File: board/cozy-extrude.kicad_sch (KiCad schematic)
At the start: 7 parts, among them J1 RPi-Pico-Socket, J2 BME280, J3 PWM-Fan, J4 Heater-Switch, K1 HF46F_5-HS1, U1 ULN2003

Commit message: improved hf46f footprint and model
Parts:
- K1: footprint Hongfa-HF46F:HF46F_5-HS1 -> Hongfa-HF46F:HF46F
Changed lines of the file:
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@@
     (property "Reference" "K1" (id 0) (at 178.435 103.505 90))
     (property "Value" "HF46F_5-HS1" (id 1) (at 179.07 106.045 90))
-    (property "Footprint" "Hongfa-HF46F:HF46F_5-HS1" (id 2) (at 190.5 97.79 0)
+    (property "Footprint" "Hongfa-HF46F:HF46F" (id 2) (at 190.5 97.79 0)
       (effects (font (size 1.27 1.27)) hide)
     )
@@
     )
     (path "/e81af6a5-45c6-4d18-ac2c-2f6d6836f747"
-      (reference "K1") (unit 1) (value "HF46F_5-HS1") (footprint "Hongfa-HF46F:HF46F_5-HS1")
+      (reference "K1") (unit 1) (value "HF46F_5-HS1") (footprint "Hongfa-HF46F:HF46F")
     )
     (path "/a47ea3c8-3841-47fd-a5b3-6e9dc298f59d"

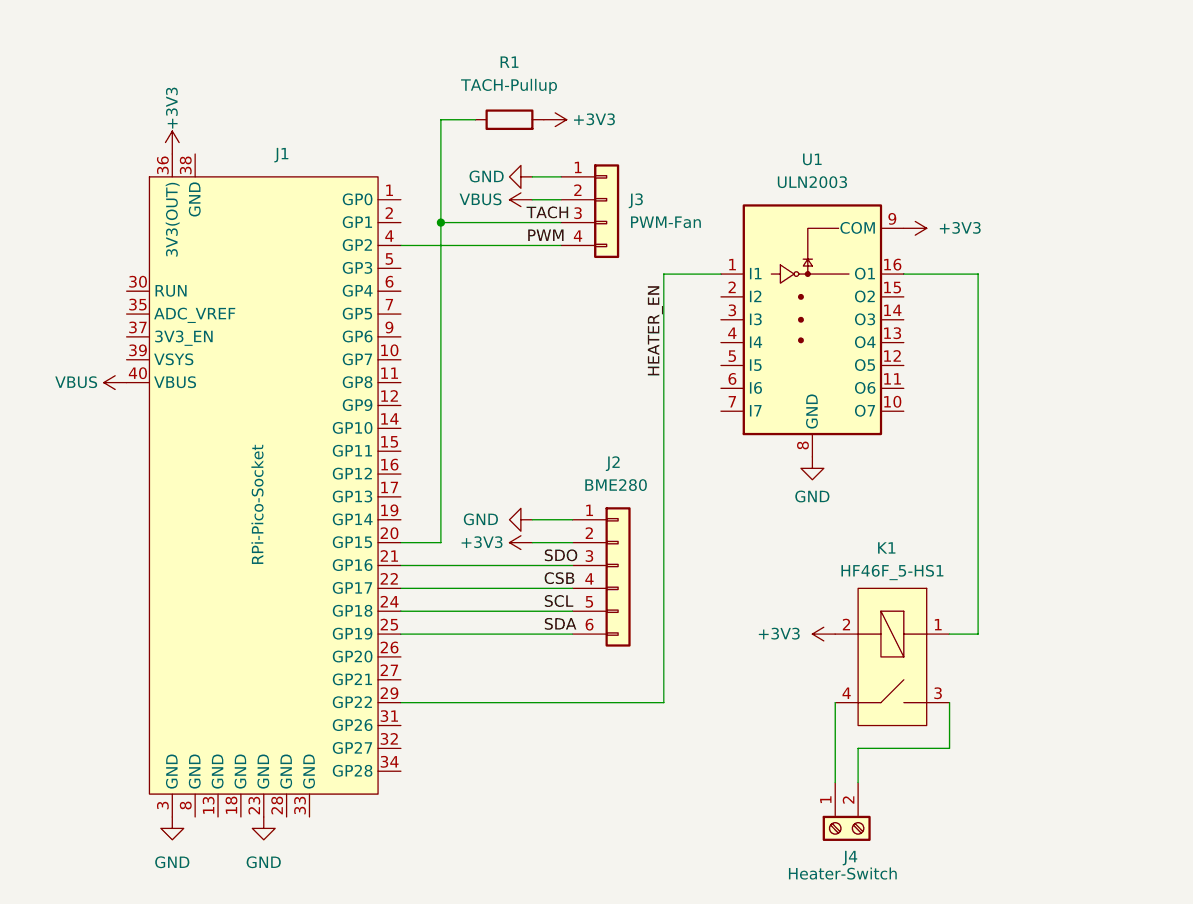
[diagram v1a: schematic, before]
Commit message: improved pcb
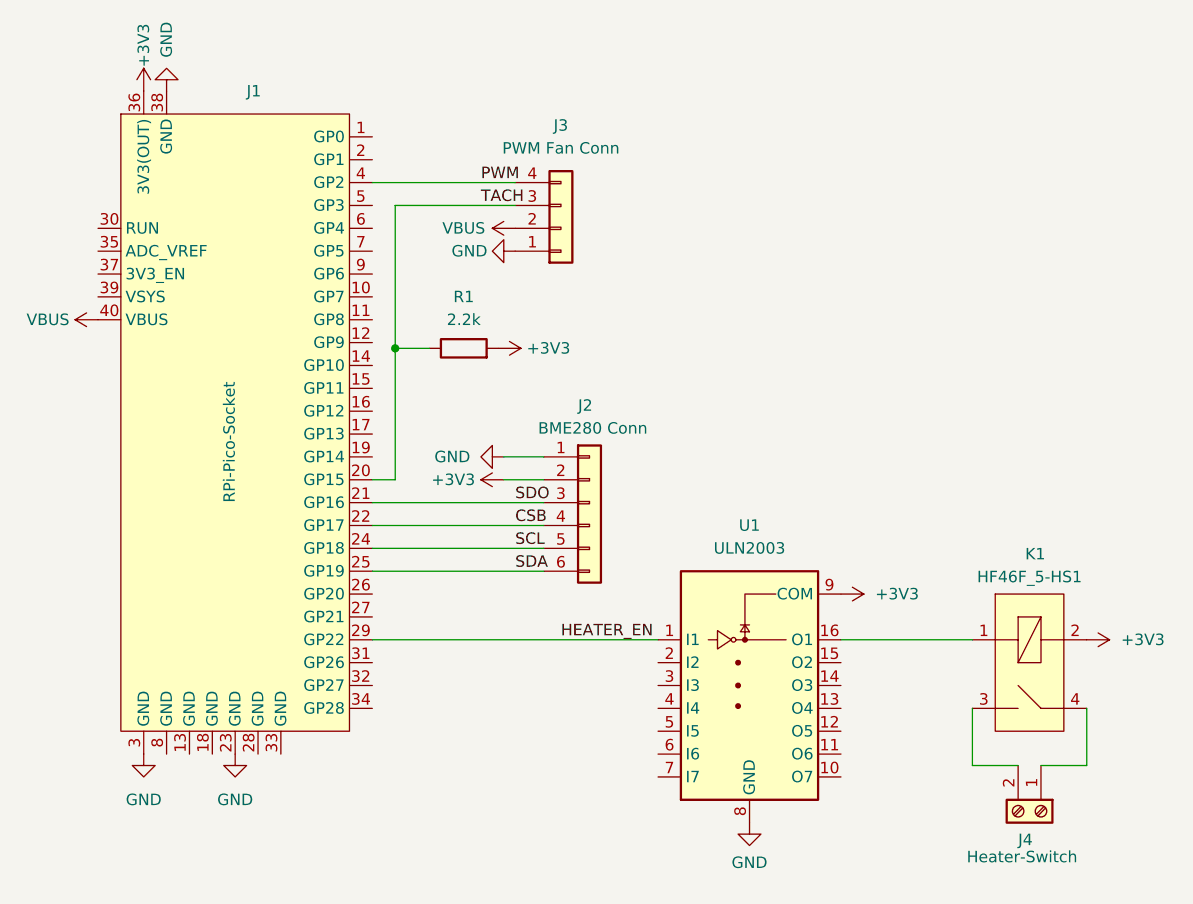
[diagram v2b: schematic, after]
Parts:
- J2: value BME280 -> BME280 Conn
- J3: value PWM-Fan -> PWM Fan Conn
- R1: value TACH-Pullup -> 2.2k
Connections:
- net GND: now also J1.38 (GND)
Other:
- moved on the sheet: J1, J2, J3, J4, K1, R1, U1
